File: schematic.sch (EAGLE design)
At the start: 30 parts, among them IC1 ATMEGA32L-8AU, IC2 7805DT, J1 POWER_JACKPTH_BREAD

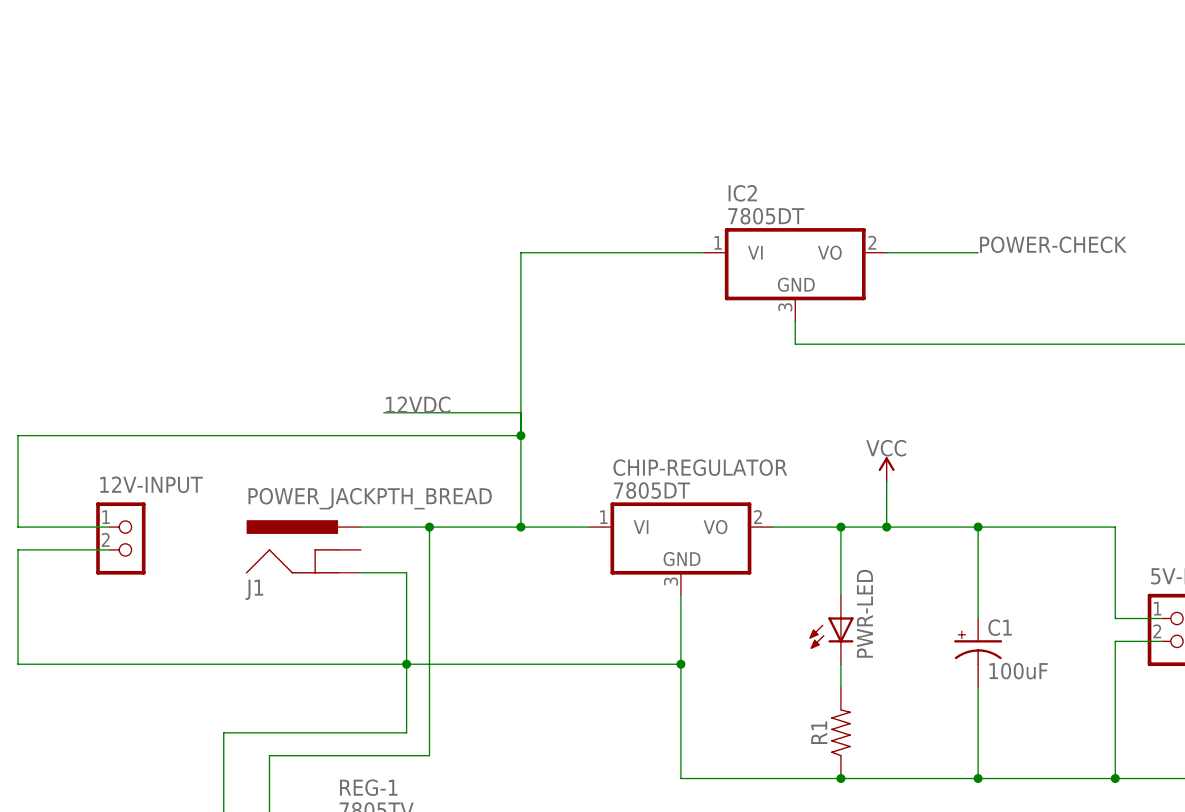
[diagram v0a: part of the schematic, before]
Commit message: Please enter the commit message for your changes. Lines starting
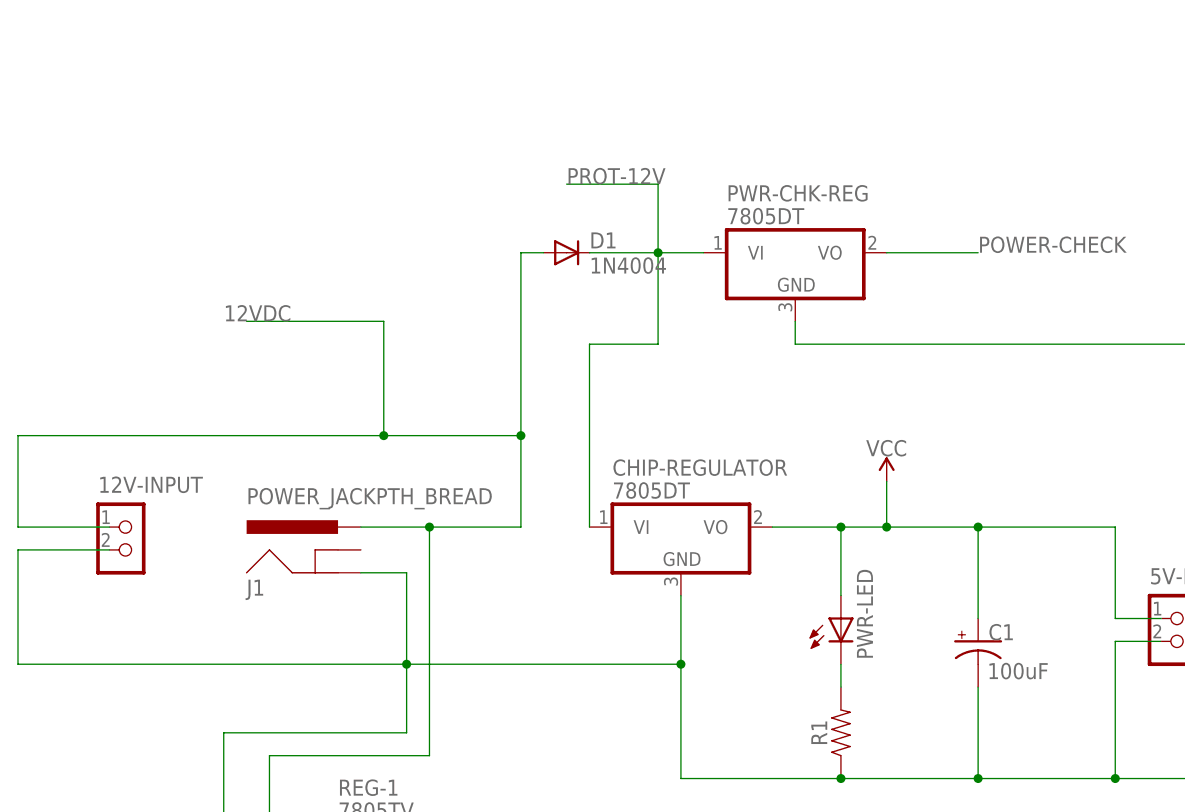
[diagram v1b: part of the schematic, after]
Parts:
- added D1: 1N4004, adafruit:1N4004
- renumbered IC2 to PWR-CHK-REG
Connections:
- new net PROT-12V: CHIP-REGULATOR.VI, D1.C, PWR-CHK-REG.VI
- net 12VDC: now also D1.A; no longer CHIP-REGULATOR.VI, PWR-CHK-REG.VI
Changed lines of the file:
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@@
 <part name="LCD1" library="SparkFun-Displays" deviceset="LCD-16X2" device="NOHOLES" override_package3d_urn="urn:adsk.eagle:package:24334248/2" override_package_urn="urn:adsk.eagle:footprint:24334249/1"/>
 <part name="J1" library="SparkFun-Connectors" deviceset="POWER_JACK" device="PTH_BREAD" override_package3d_urn="urn:adsk.eagle:package:24334302/2" override_package_urn="urn:adsk.eagle:footprint:24334303/1"/>
-<part name="VALVES-SUPPLY" library="con-phoenix-508" library_urn="urn:adsk.eagle:library:176" deviceset="MSTBA8" device="" package3d_urn="urn:adsk.eagle:package:9620/1">
+<part name="VALVES-SUPPLY" library="con-phoenix-508" library_urn="urn:adsk.eagle:library:176" deviceset="MSTBA8" device="" package3d_urn="urn:adsk.eagle:package:9620/1" override_package3d_urn="urn:adsk.eagle:package:24339764/2" override_package_urn="urn:adsk.eagle:footprint:9526/1">
 <attribute name="SPICEPREFIX" value="X"/>
 </part>
@@
 <part name="R4" library="SparkFun-Resistors" deviceset="RESISTOR" device="1206" override_package3d_urn="urn:adsk.eagle:package:24334298/2" override_package_urn="urn:adsk.eagle:footprint:24334299/1" value=" "/>
 <part name="R6" library="SparkFun-Resistors" deviceset="RESISTOR" device="1206" value=" "/>
-<part name="VALVE" library="con-phoenix-508" library_urn="urn:adsk.eagle:library:176" deviceset="MSTBA6" device="" package3d_urn="urn:adsk.eagle:package:9616/1"/>
-<part name="COMMON-GND" library="con-phoenix-508" library_urn="urn:adsk.eagle:library:176" deviceset="MSTBA6" device="" package3d_urn="urn:adsk.eagle:package:9616/1"/>
-<part name="5V-SUPPLY" library="con-phoenix-508" library_urn="urn:adsk.eagle:library:176" deviceset="MSTBA6" device="" package3d_urn="urn:adsk.eagle:package:9616/1"/>
+<part name="VALVE" library="con-phoenix-508" library_urn="urn:adsk.eagle:library:176" deviceset="MSTBA6" device="" package3d_urn="urn:adsk.eagle:package:9616/1" override_package3d_urn="urn:adsk.eagle:package:24339798/2" override_package_urn="urn:adsk.eagle:footprint:9524/1"/>
+<part name="COMMON-GND" library="con-phoenix-508" library_urn="urn:adsk.eagle:library:176" deviceset="MSTBA6" device="" package3d_urn="urn:adsk.eagle:package:9616/1" override_package3d_urn="urn:adsk.eagle:package:24339781/2" override_package_urn="urn:adsk.eagle:footprint:9524/1"/>
+<part name="5V-SUPPLY" library="con-phoenix-508" library_urn="urn:adsk.eagle:library:176" deviceset="MSTBA6" device="" package3d_urn="urn:adsk.eagle:package:9616/1" override_package3d_urn="urn:adsk.eagle:package:24339787/2" override_package_urn="urn:adsk.eagle:footprint:9524/1"/>
 <part name="ISP-HEADER" library="SparkFun-Connectors" deviceset="AVR_SPI_PROG_3X2" device="NS" override_package3d_urn="urn:adsk.eagle:package:24334515/2" override_package_urn="urn:adsk.eagle:footprint:24334516/1"/>
-<part name="VALVES-GND" library="con-phoenix-508" library_urn="urn:adsk.eagle:library:176" deviceset="MSTBA8" device="" package3d_urn="urn:adsk.eagle:package:9620/1"/>
+<part name="VALVES-GND" library="con-phoenix-508" library_urn="urn:adsk.eagle:library:176" deviceset="MSTBA8" device="" package3d_urn="urn:adsk.eagle:package:9620/1" override_package3d_urn="urn:adsk.eagle:package:24339756/2" override_package_urn="urn:adsk.eagle:footprint:9526/1"/>
 <part name="REG-1" library="linear" library_urn="urn:adsk.eagle:library:262" deviceset="78*" device="TV" package3d_urn="urn:adsk.eagle:package:16417/2" technology="05"/>
 <part name="REG-2" library="linear" library_urn="urn:adsk.eagle:library:262" deviceset="78*" device="TV" package3d_urn="urn:adsk.eagle:package:16417/2" technology="05"/>
@@
 <part name="12V-INPUT" library="dp_devices" deviceset="CON_TERMINAL_BLOCK_02" device="-5MM" override_package3d_urn="urn:adsk.eagle:package:24334674/2" override_package_urn="urn:adsk.eagle:footprint:24334675/1"/>
 <part name="DEBUG" library="adafruit" deviceset="PINHD-1X6" device="B" override_package3d_urn="urn:adsk.eagle:package:24334676/2" override_package_urn="urn:adsk.eagle:footprint:24334677/1"/>
-<part name="C1" library="SparkFun-Capacitors" deviceset="100UF-POLAR" device="-RADIAL-2.5MM-25V-20%" value="100uF"/>
-<part name="IC2" library="adafruit" deviceset="78*" device="DT" technology="05"/>
+<part name="C1" library="SparkFun-Capacitors" deviceset="100UF-POLAR" device="-RADIAL-2.5MM-25V-20%" override_package3d_urn="urn:adsk.eagle:package:24339134/2" override_package_urn="urn:adsk.eagle:footprint:24339135/1" value="100uF"/>
+<part name="PWR-CHK-REG" library="adafruit" deviceset="78*" device="DT" override_package3d_urn="urn:adsk.eagle:package:24339171/2" override_package_urn="urn:adsk.eagle:footprint:24339173/1" technology="05"/>
+<part name="D1" library="adafruit" deviceset="1N4004" device="" override_package3d_urn="urn:adsk.eagle:package:24340694/2" override_package_urn="urn:adsk.eagle:footprint:24340695/1"/>
 </parts>
 <sheets>
@@
 </instance>
 <instance part="C1" gate="G$1" x="-43.18" y="124.46" smashed="yes">
-<attribute name="NAME" x="-42.164" y="125.095" size="1.778" layer="95" font="vector"/>
+<attribute name="NAME" x="-39.116" y="126.365" size="1.778" layer="95" font="vector" rot="R180"/>
 <attribute name="VALUE" x="-42.164" y="120.269" size="1.778" layer="96" font="vector"/>
 </instance>
-<instance part="IC2" gate="A1" x="-63.5" y="167.64" smashed="yes">
+<instance part="PWR-CHK-REG" gate="A1" x="-63.5" y="167.64" smashed="yes">
 <attribute name="NAME" x="-71.12" y="173.355" size="1.778" layer="95"/>
 <attribute name="VALUE" x="-71.12" y="170.815" size="1.778" layer="96"/>
+</instance>
+<instance part="D1" gate="1" x="-88.9" y="167.64" smashed="yes">
+<attribute name="NAME" x="-86.36" y="168.1226" size="1.778" layer="95"/>
+<attribute name="VALUE" x="-86.36" y="165.3286" size="1.778" layer="96"/>
 </instance>
 </instances>
@@
 <segment>
 <pinref part="J1" gate="G$1" pin="PWR"/>
-<pinref part="CHIP-REGULATOR" gate="A1" pin="VI"/>
 <wire x1="-111.76" y1="137.16" x2="-104.14" y2="137.16" width="0.1524" layer="91"/>
 <wire x1="-104.14" y1="137.16" x2="-93.98" y2="137.16" width="0.1524" layer="91"/>
-<wire x1="-93.98" y1="137.16" x2="-86.36" y2="137.16" width="0.1524" layer="91"/>
 <wire x1="-104.14" y1="137.16" x2="-104.14" y2="111.76" width="0.1524" layer="91"/>
 <junction x="-104.14" y="137.16"/>
 <wire x1="-104.14" y1="111.76" x2="-121.92" y2="111.76" width="0.1524" layer="91"/>
 <wire x1="-93.98" y1="137.16" x2="-93.98" y2="147.32" width="0.1524" layer="91"/>
-<junction x="-93.98" y="137.16"/>
-<wire x1="-93.98" y1="147.32" x2="-93.98" y2="149.86" width="0.1524" layer="91"/>
-<wire x1="-93.98" y1="149.86" x2="-109.22" y2="149.86" width="0.1524" layer="91"/>
-<label x="-109.22" y="149.86" size="1.778" layer="95"/>
 <wire x1="-121.92" y1="111.76" x2="-121.92" y2="101.6" width="0.1524" layer="91"/>
 <pinref part="REG-1" gate="A1" pin="VI"/>
@@
 <wire x1="-139.7" y1="137.16" x2="-149.86" y2="137.16" width="0.1524" layer="91"/>
 <wire x1="-149.86" y1="137.16" x2="-149.86" y2="147.32" width="0.1524" layer="91"/>
-<wire x1="-149.86" y1="147.32" x2="-93.98" y2="147.32" width="0.1524" layer="91"/>
+<wire x1="-149.86" y1="147.32" x2="-109.22" y2="147.32" width="0.1524" layer="91"/>
 <junction x="-93.98" y="147.32"/>
-<pinref part="IC2" gate="A1" pin="VI"/>
-<wire x1="-73.66" y1="167.64" x2="-93.98" y2="167.64" width="0.1524" layer="91"/>
+<wire x1="-109.22" y1="147.32" x2="-93.98" y2="147.32" width="0.1524" layer="91"/>
 <wire x1="-93.98" y1="167.64" x2="-93.98" y2="147.32" width="0.1524" layer="91"/>
+<wire x1="-109.22" y1="160.02" x2="-124.46" y2="160.02" width="0.1524" layer="91"/>
+<label x="-127" y="160.02" size="1.778" layer="95"/>
+<wire x1="-109.22" y1="160.02" x2="-109.22" y2="147.32" width="0.1524" layer="91"/>
+<junction x="-109.22" y="147.32"/>
+<pinref part="D1" gate="1" pin="A"/>
+<wire x1="-93.98" y1="167.64" x2="-91.44" y2="167.64" width="0.1524" layer="91"/>
 </segment>
 <segment>
@@
 <wire x1="-43.18" y1="119.38" x2="-43.18" y2="109.22" width="0.1524" layer="91"/>
 <junction x="-43.18" y="109.22"/>
-<pinref part="IC2" gate="A1" pin="GND"/>
+<pinref part="PWR-CHK-REG" gate="A1" pin="GND"/>
 <wire x1="-63.5" y1="160.02" x2="-63.5" y2="157.48" width="0.1524" layer="91"/>
 <wire x1="-63.5" y1="157.48" x2="-12.7" y2="157.48" width="0.1524" layer="91"/>
@@
 <net name="POWER-CHECK" class="0">
 <segment>
-<pinref part="IC2" gate="A1" pin="VO"/>
+<pinref part="PWR-CHK-REG" gate="A1" pin="VO"/>
 <wire x1="-53.34" y1="167.64" x2="-43.18" y2="167.64" width="0.1524" layer="91"/>
 <label x="-43.18" y="167.64" size="1.778" layer="95"/>
@@
 </segment>
 </net>
+<net name="PROT-12V" class="0">
+<segment>
+<pinref part="D1" gate="1" pin="C"/>
+<pinref part="PWR-CHK-REG" gate="A1" pin="VI"/>
+<wire x1="-86.36" y1="167.64" x2="-78.74" y2="167.64" width="0.1524" layer="91"/>
+<pinref part="CHIP-REGULATOR" gate="A1" pin="VI"/>
+<wire x1="-78.74" y1="167.64" x2="-73.66" y2="167.64" width="0.1524" layer="91"/>
+<wire x1="-86.36" y1="137.16" x2="-86.36" y2="157.48" width="0.1524" layer="91"/>
+<wire x1="-86.36" y1="157.48" x2="-78.74" y2="157.48" width="0.1524" layer="91"/>
+<wire x1="-78.74" y1="157.48" x2="-78.74" y2="167.64" width="0.1524" layer="91"/>
+<junction x="-78.74" y="167.64"/>
+<wire x1="-78.74" y1="167.64" x2="-78.74" y2="175.26" width="0.1524" layer="91"/>
+<wire x1="-78.74" y1="175.26" x2="-88.9" y2="175.26" width="0.1524" layer="91"/>
+<label x="-88.9" y="175.26" size="1.778" layer="95"/>
+</segment>
+</net>
